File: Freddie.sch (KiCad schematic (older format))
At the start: 22 parts, among them J3 Cartridge, U10 74LS08, U13 74LS138, U14 MMU, U9 Freddie, Y1 14,18757MHz

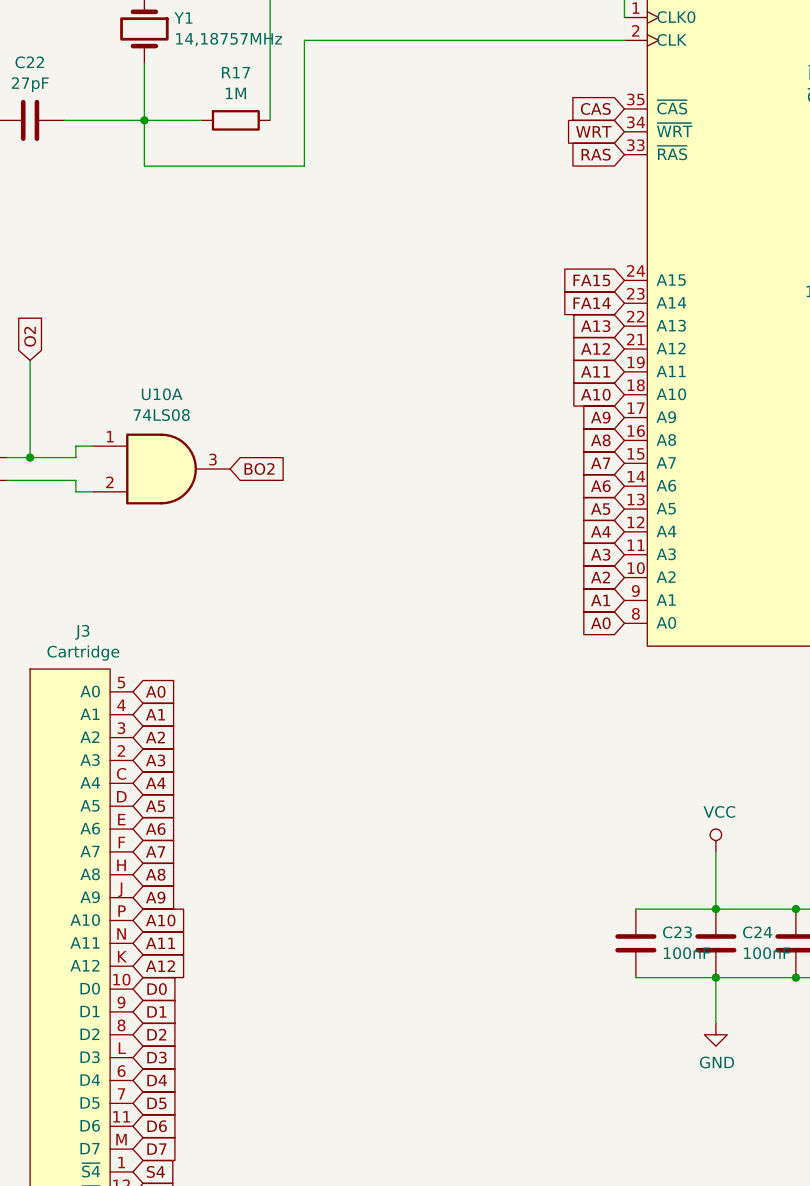
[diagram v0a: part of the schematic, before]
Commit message: Finished GND
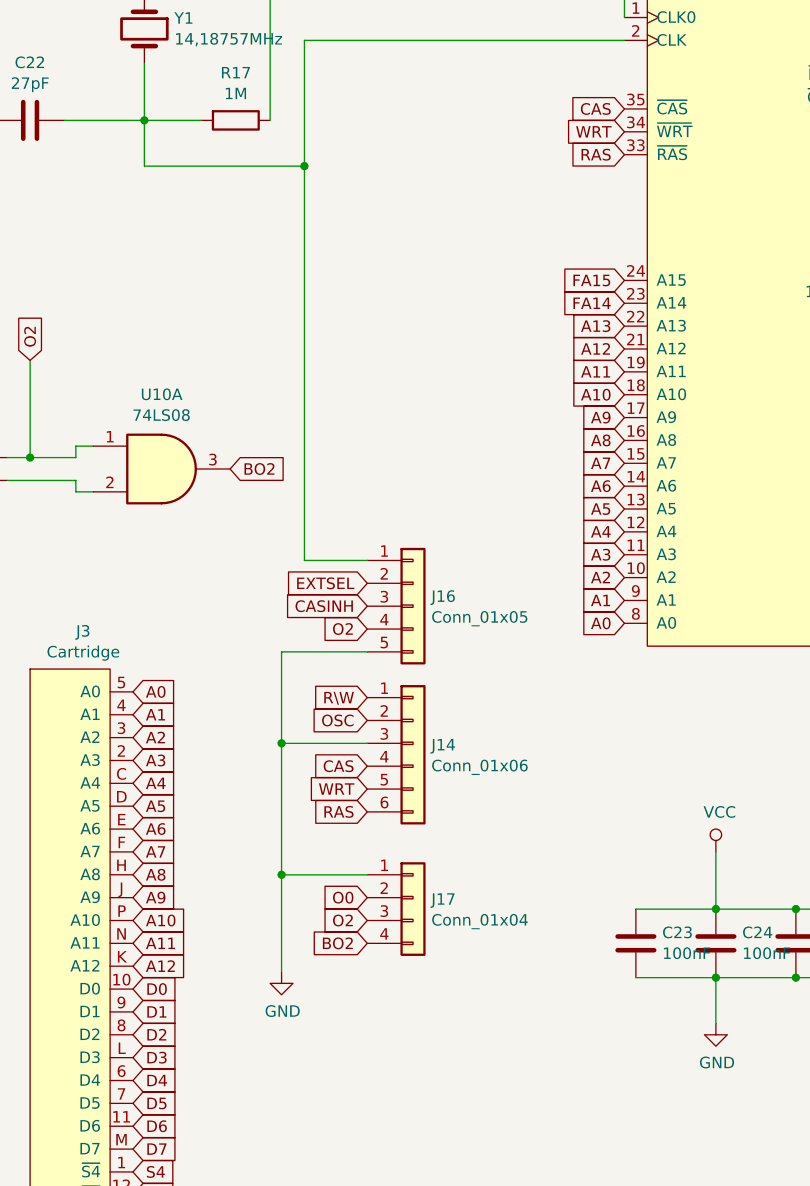
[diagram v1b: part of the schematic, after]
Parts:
- added J14: Conn_01x06, Connector_PinHeader_2.54mm:PinHeader_1x06_P2.54mm_Vertical, symbol Connector_Generic:Conn_01x06
- added J16: Conn_01x05, Connector_PinHeader_2.54mm:PinHeader_1x05_P2.54mm_Vertical, symbol Connector_Generic:Conn_01x05
- added J17: Conn_01x04, Connector_PinHeader_2.54mm:PinHeader_1x04_P2.54mm_Vertical, symbol Connector_Generic:Conn_01x04
- R16, R17: footprint Resistor_THT:R_Axial_DIN0207_L6.3mm_D2.5mm_P10.16mm_Horizontal -> Atari:R_Axial_DIN0207_L3.6mm_D2.2mm_P10.16mm_Horizontal
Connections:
- net BO2: now also J17.4 (Pin_4)
- net CAS: now also J14.4 (Pin_4)
- net CASINH: now also J16.3 (Pin_3)
- net EXTSEL: now also J16.2 (Pin_2)
- net GND: now also J14.3 (Pin_3), J16.5 (Pin_5), J17.1 (Pin_1)
- net O2: now also J16.4 (Pin_4), J17.3 (Pin_3)
- net OSC: now also J14.2 (Pin_2)
- net RAS: now also J14.6 (Pin_6)
- net R\W: now also J14.1 (Pin_1)
- net WRT: now also J14.5 (Pin_5)
- net at C22.1, R17.2, U9.2 (CLK)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: now also J16.1 (Pin_1)
- new net O0: J17.2 (Pin_2)
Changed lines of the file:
@@
 F 0 "R16" V 2143 1250 50  0000 C CNN
 F 1 "240" V 2234 1250 50  0000 C CNN
-F 2 "Resistor_THT:R_Axial_DIN0207_L6.3mm_D2.5mm_P10.16mm_Horizontal" V 2280 1250 50  0001 C CNN
+F 2 "Atari:R_Axial_DIN0207_L3.6mm_D2.2mm_P10.16mm_Horizontal" V 2280 1250 50  0001 C CNN
 F 3 "~" H 2350 1250 50  0001 C CNN
 	1    2350 1250
@@
 F 0 "R17" V 2143 2000 50  0000 C CNN
 F 1 "1M" V 2234 2000 50  0000 C CNN
-F 2 "Resistor_THT:R_Axial_DIN0207_L6.3mm_D2.5mm_P10.16mm_Horizontal" V 2280 2000 50  0001 C CNN
+F 2 "Atari:R_Axial_DIN0207_L3.6mm_D2.2mm_P10.16mm_Horizontal" V 2280 2000 50  0001 C CNN
 F 3 "~" H 2350 2000 50  0001 C CNN
 	1    2350 2000
@@
 	9500 1800 9550 1800
 Connection ~ 9500 1700
+$Comp
+L Connector_Generic:Conn_01x06 J14
+U 1 1 5FC9F389
+P 3125 4725
+F 0 "J14" H 3205 4717 50  0000 L CNN
+F 1 "Conn_01x06" H 3205 4626 50  0000 L CNN
+F 2 "Connector_PinHeader_2.54mm:PinHeader_1x06_P2.54mm_Vertical" H 3125 4725 50  0001 C CNN
+F 3 "~" H 3125 4725 50  0001 C CNN
+	1    3125 4725
+	1    0    0    -1
+$EndComp
+Text GLabel 2925 4525 0    50   Input ~ 0
+R\W
+Text GLabel 2925 4625 0    50   Input ~ 0
+OSC
+Text GLabel 2925 4825 0    50   Input ~ 0
+CAS
+Text GLabel 2925 4925 0    50   Input ~ 0
+WRT
+Text GLabel 2925 5025 0    50   Input ~ 0
+RAS
+$Comp
+L power:GND #PWR0128
+U 1 1 5FCA0518
+P 2550 5725
+F 0 "#PWR0128" H 2550 5475 50  0001 C CNN
+F 1 "GND" H 2555 5552 50  0000 C CNN
+F 2 "" H 2550 5725 50  0001 C CNN
+F 3 "" H 2550 5725 50  0001 C CNN
+	1    2550 5725
+	1    0    0    -1
+$EndComp
+Wire Wire Line
+	2925 4725 2550 4725
+$Comp
+L Connector_Generic:Conn_01x05 J16
+U 1 1 5FCAEA58
+P 3125 4125
+F 0 "J16" H 3205 4167 50  0000 L CNN
+F 1 "Conn_01x05" H 3205 4076 50  0000 L CNN
+F 2 "Connector_PinHeader_2.54mm:PinHeader_1x05_P2.54mm_Vertical" H 3125 4125 50  0001 C CNN
+F 3 "~" H 3125 4125 50  0001 C CNN
+	1    3125 4125
+	1    0    0    -1
+$EndComp
+Wire Wire Line
+	2650 2200 2650 3925
+Wire Wire Line
+	2650 3925 2925 3925
+Connection ~ 2650 2200
+Text GLabel 2925 4025 0    50   Input ~ 0
+EXTSEL
+Text GLabel 2925 4125 0    50   Input ~ 0
+CASINH
+Text GLabel 2925 4225 0    50   Input ~ 0
+O2
+Wire Wire Line
+	2925 4325 2550 4325
+Wire Wire Line
+	2550 4325 2550 4725
+Connection ~ 2550 4725
+$Comp
+L Connector_Generic:Conn_01x04 J17
+U 1 1 5FCBC25F
+P 3125 5400
+F 0 "J17" H 3205 5392 50  0000 L CNN
+F 1 "Conn_01x04" H 3205 5301 50  0000 L CNN
+F 2 "Connector_PinHeader_2.54mm:PinHeader_1x04_P2.54mm_Vertical" H 3125 5400 50  0001 C CNN
+F 3 "~" H 3125 5400 50  0001 C CNN
+	1    3125 5400
+	1    0    0    -1
+$EndComp
+Wire Wire Line
+	2550 4725 2550 5300
+Text GLabel 2925 5400 0    50   Input ~ 0
+O0
+Text GLabel 2925 5600 0    50   Input ~ 0
+BO2
+Text GLabel 2925 5500 0    50   Input ~ 0
+O2
+Wire Wire Line
+	2925 5300 2550 5300
+Connection ~ 2550 5300
+Wire Wire Line
+	2550 5300 2550 5725
 $EndSCHEMATC

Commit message: Gerber
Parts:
- R1: footprint Resistor_SMD:R_1206_3216Metric_Pad1.42x1.75mm_HandSolder -> Atari:R_Axial_DIN0207_L3.6mm_D2.2mm_P10.16mm_Horizontal
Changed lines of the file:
@@
 F 0 "R1" H 6130 1554 50  0000 R CNN
 F 1 "3k" H 6130 1645 50  0000 R CNN
-F 2 "Resistor_SMD:R_1206_3216Metric_Pad1.42x1.75mm_HandSolder" V 6130 1600 50  0001 C CNN
+F 2 "Atari:R_Axial_DIN0207_L3.6mm_D2.2mm_P10.16mm_Horizontal" V 6130 1600 50  0001 C CNN
 F 3 "~" H 6200 1600 50  0001 C CNN
 	1    6200 1600
